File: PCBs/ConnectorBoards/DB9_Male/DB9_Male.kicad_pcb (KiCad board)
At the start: 2 copper layers, 4 parts, among them J1 DB9_Male, J2 Conn_02x05_Odd_Even

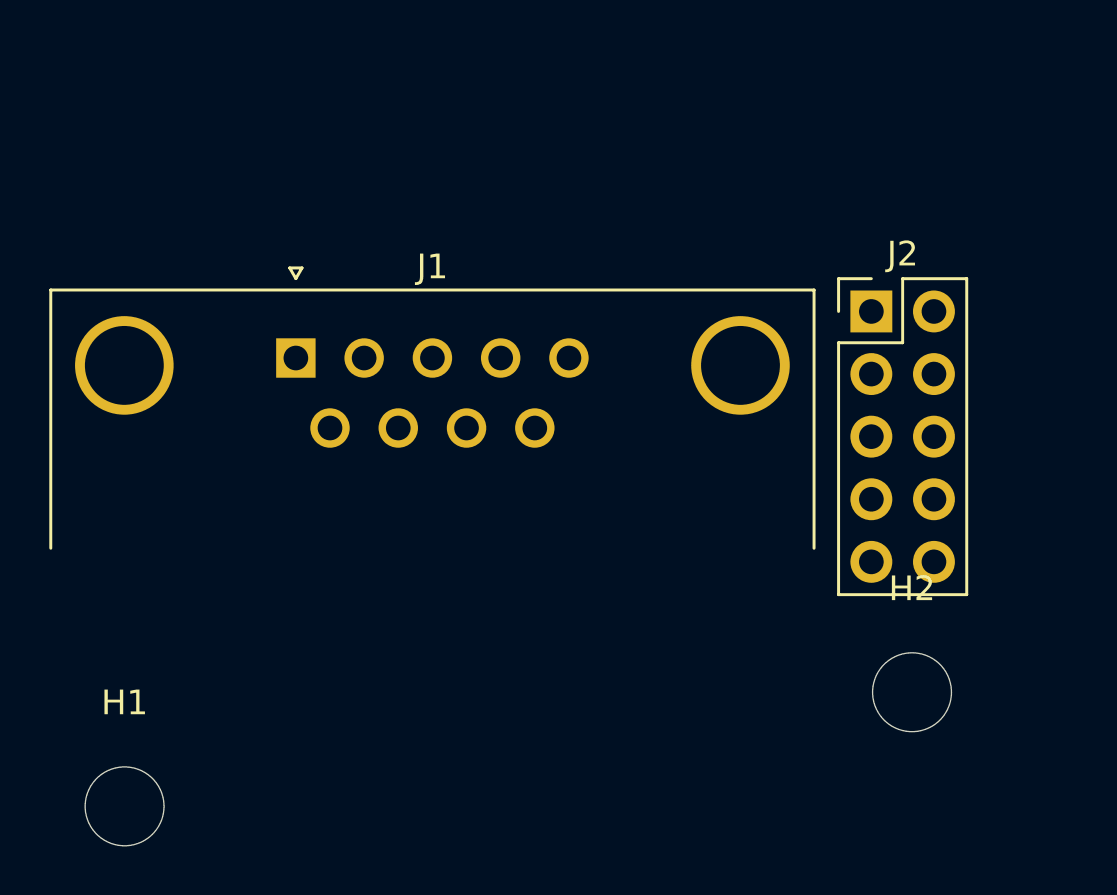
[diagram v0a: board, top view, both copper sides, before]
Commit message: generated the male pcbs
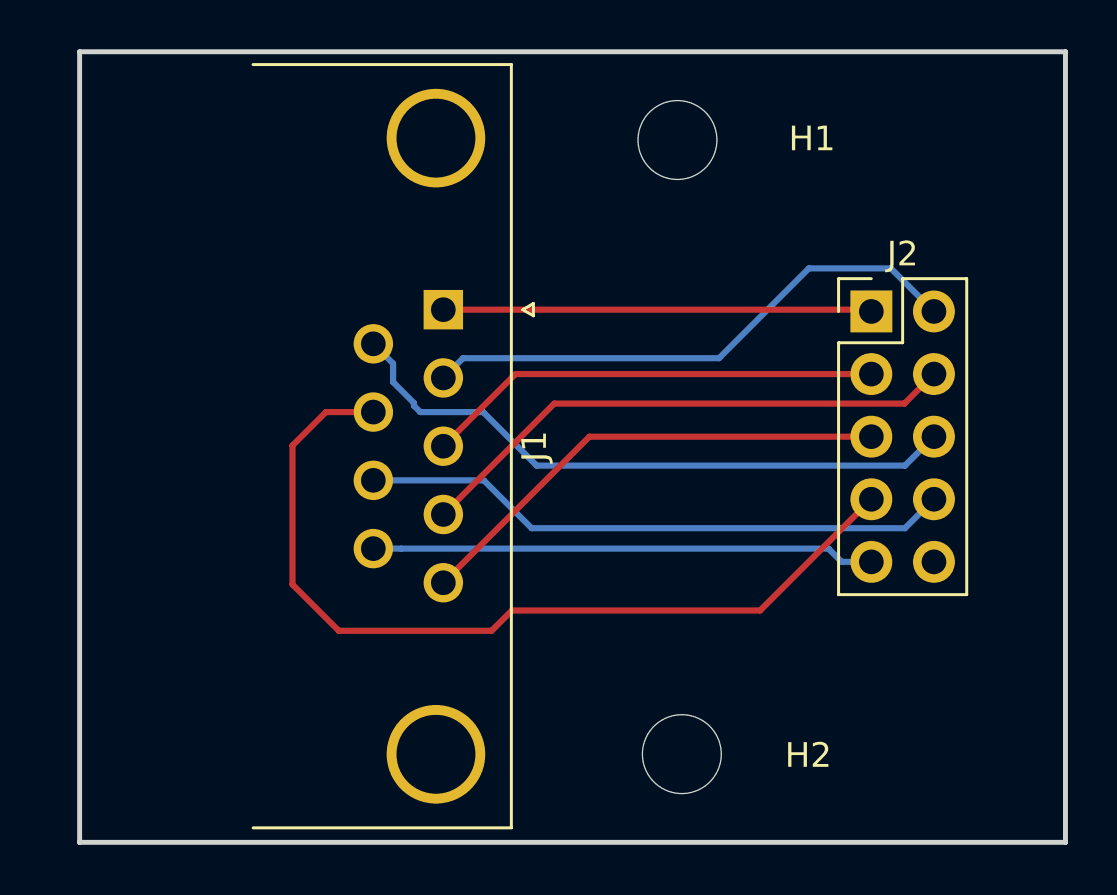
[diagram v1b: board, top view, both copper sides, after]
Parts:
- moved H1 35.1 mm to (167.1, 41.5)
- moved H2 9.67 mm to (167.3, 66.4)
- moved J1 6.30 mm to (157.6, 48.4), turned to 270 degrees
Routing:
- net 7: track 0.00 -> 36.0 mm
- net 6: track 0.00 -> 25.8 mm
- net 8: track 0.00 -> 24.0 mm
- net 2: track 0.00 -> 22.5 mm
- net 4: track 0.00 -> 22.3 mm
- net 9: track 0.00 -> 20.4 mm
- net 5: track 0.00 -> 19.8 mm
- net 3: track 0.00 -> 18.6 mm
- net 1: track 0.00 -> 17.4 mm
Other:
- board outline added: 40 x 32.1 mm
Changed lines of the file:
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@@
   (general
     (thickness 1.6)
-    (drawings 0)
-    (tracks 0)
+    (drawings 4)
+    (tracks 39)
     (zones 0)
     (modules 4)
@@
       (outputformat 1)
       (mirror false)
-      (drillshape 1)
+      (drillshape 0)
       (scaleselection 1)
-      (outputdirectory ""))
+      (outputdirectory "gerbers/"))
   )
   (net 0 "")
@@
   )
   (module MountingHole:MountingHole_3.2mm_M3 (layer F.Cu)
-    (at 144.673601 68.539401)
+    (at 167.1066 41.5036)
     (descr "Mounting Hole 3.2mm, no annular, M3")
     (tags "mounting hole 3.2mm no annular m3")
     (attr virtual)
-    (fp_text reference H1 (at 0 -4.2) (layer F.SilkS)
+    (fp_text reference H1 (at 5.461 -0.0508) (layer F.SilkS)
       (effects (font (size 1 1) (thickness 0.15)))
     )
@@
   )
   (module MountingHole:MountingHole_3.2mm_M3 (layer F.Cu)
-    (at 176.623601 63.909401)
+    (at 167.2844 66.421)
     (descr "Mounting Hole 3.2mm, no annular, M3")
     (tags "mounting hole 3.2mm no annular m3")
     (attr virtual)
-    (fp_text reference H2 (at 0 -4.2) (layer F.SilkS)
+    (fp_text reference H2 (at 5.1308 0.0508) (layer F.SilkS)
       (effects (font (size 1 1) (thickness 0.15)))
     )
@@
   )
   (module Connector_Dsub:DSUB-9_Male_Horizontal_P2.77x2.84mm_EdgePinOffset4.94mm_Housed_MountingHolesOffset7.48mm (layer F.Cu)
-    (at 151.623601 50.348739)
+    (at 157.607 48.387 270)
     (descr "9-pin D-Sub connector, horizontal/angled (90 deg), THT-mount, male, pitch 2.77x2.84mm, pin-PCB-offset 4.9399999999999995mm, distance of mounting holes 25mm, distance of mounting holes to PCB edge 7.4799999999999995mm, see https://disti-assets.s3.amazonaws.com/tonar/files/datasheets/16730.pdf")
     (tags "9-pin D-Sub connector horizontal angled 90deg THT male pitch 2.77x2.84mm pin-PCB-offset 4.9399999999999995mm mounting-holes-distance 25mm mounting-hole-offset 25mm")
-    (fp_text reference J1 (at 5.54 -3.7) (layer F.SilkS)
-      (effects (font (size 1 1) (thickness 0.15)))
-    )
-    (fp_text value DB9_Male (at 5.54 15.68) (layer F.Fab)
+    (fp_text reference J1 (at 5.54 -3.7 270) (layer F.SilkS)
+      (effects (font (size 1 1) (thickness 0.15)))
+    )
+    (fp_text value DB9_Male (at 5.54 15.68 270) (layer F.Fab)
       (effects (font (size 1 1) (thickness 0.15)))
     )
@@
     (fp_line (start 21.5 14.7) (end 21.5 -3.25) (layer F.CrtYd) (width 0.05))
     (fp_line (start 21.5 -3.25) (end -10.4 -3.25) (layer F.CrtYd) (width 0.05))
-    (fp_text user %R (at 5.54 11.18) (layer F.Fab)
-      (effects (font (size 1 1) (thickness 0.15)))
-    )
-    (pad 1 thru_hole rect (at 0 0) (size 1.6 1.6) (drill 1) (layers *.Cu *.Mask)
+    (fp_text user %R (at 5.54 11.18 270) (layer F.Fab)
+      (effects (font (size 1 1) (thickness 0.15)))
+    )
+    (pad 1 thru_hole rect (at 0 0 270) (size 1.6 1.6) (drill 1) (layers *.Cu *.Mask)
       (net 1 1))
-    (pad 2 thru_hole circle (at 2.77 0) (size 1.6 1.6) (drill 1) (layers *.Cu *.Mask)
+    (pad 2 thru_hole circle (at 2.77 0 270) (size 1.6 1.6) (drill 1) (layers *.Cu *.Mask)
       (net 2 2))
-    (pad 3 thru_hole circle (at 5.54 0) (size 1.6 1.6) (drill 1) (layers *.Cu *.Mask)
+    (pad 3 thru_hole circle (at 5.54 0 270) (size 1.6 1.6) (drill 1) (layers *.Cu *.Mask)
       (net 3 3))
-    (pad 4 thru_hole circle (at 8.31 0) (size 1.6 1.6) (drill 1) (layers *.Cu *.Mask)
+    (pad 4 thru_hole circle (at 8.31 0 270) (size 1.6 1.6) (drill 1) (layers *.Cu *.Mask)
       (net 4 4))
-    (pad 5 thru_hole circle (at 11.08 0) (size 1.6 1.6) (drill 1) (layers *.Cu *.Mask)
+    (pad 5 thru_hole circle (at 11.08 0 270) (size 1.6 1.6) (drill 1) (layers *.Cu *.Mask)
       (net 5 5))
-    (pad 6 thru_hole circle (at 1.385 2.84) (size 1.6 1.6) (drill 1) (layers *.Cu *.Mask)
+    (pad 6 thru_hole circle (at 1.385 2.84 270) (size 1.6 1.6) (drill 1) (layers *.Cu *.Mask)
       (net 6 6))
-    (pad 7 thru_hole circle (at 4.155 2.84) (size 1.6 1.6) (drill 1) (layers *.Cu *.Mask)
+    (pad 7 thru_hole circle (at 4.155 2.84 270) (size 1.6 1.6) (drill 1) (layers *.Cu *.Mask)
       (net 7 7))
-    (pad 8 thru_hole circle (at 6.925 2.84) (size 1.6 1.6) (drill 1) (layers *.Cu *.Mask)
+    (pad 8 thru_hole circle (at 6.925 2.84 270) (size 1.6 1.6) (drill 1) (layers *.Cu *.Mask)
       (net 8 8))
-    (pad 9 thru_hole circle (at 9.695 2.84) (size 1.6 1.6) (drill 1) (layers *.Cu *.Mask)
+    (pad 9 thru_hole circle (at 9.695 2.84 270) (size 1.6 1.6) (drill 1) (layers *.Cu *.Mask)
       (net 9 9))
-    (pad 0 thru_hole circle (at -6.96 0.3) (size 4 4) (drill 3.2) (layers *.Cu *.Mask))
-    (pad 0 thru_hole circle (at 18.04 0.3) (size 4 4) (drill 3.2) (layers *.Cu *.Mask))
+    (pad 0 thru_hole circle (at -6.96 0.3 270) (size 4 4) (drill 3.2) (layers *.Cu *.Mask))
+    (pad 0 thru_hole circle (at 18.04 0.3 270) (size 4 4) (drill 3.2) (layers *.Cu *.Mask))
     (model ${KISYS3DMOD}/Connector_Dsub.3dshapes/DSUB-9_Male_Horizontal_P2.77x2.84mm_EdgePinOffset4.94mm_Housed_MountingHolesOffset7.48mm.wrl
       (at (xyz 0 0 0))
@@
     )
   )
+  (gr_line (start 142.8496 37.9222) (end 142.8496 70) (layer Edge.Cuts) (width 0.2))
+  (gr_line (start 182.8496 37.9222) (end 142.8496 37.9222) (layer Edge.Cuts) (width 0.2))
+  (gr_line (start 182.8496 70) (end 182.8496 37.9222) (layer Edge.Cuts) (width 0.2))
+  (gr_line (start 142.8496 70) (end 182.8496 70) (layer Edge.Cuts) (width 0.2))
+  (segment (start 174.9012 48.387) (end 174.973601 48.459401) (width 0.25) (layer F.Cu) (net 1))
+  (segment (start 157.607 48.387) (end 174.9012 48.387) (width 0.25) (layer F.Cu) (net 1))
+  (segment (start 158.406999 50.357001) (end 168.794199 50.357001) (width 0.25) (layer B.Cu) (net 2))
+  (segment (start 157.607 51.157) (end 158.406999 50.357001) (width 0.25) (layer B.Cu) (net 2))
+  (segment (start 168.794199 50.357001) (end 172.4406 46.7106) (width 0.25) (layer B.Cu) (net 2))
+  (segment (start 175.7648 46.7106) (end 177.513601 48.459401) (width 0.25) (layer B.Cu) (net 2))
+  (segment (start 172.4406 46.7106) (end 175.7648 46.7106) (width 0.25) (layer B.Cu) (net 2))
+  (segment (start 160.534599 50.999401) (end 157.607 53.927) (width 0.25) (layer F.Cu) (net 3))
+  (segment (start 174.973601 50.999401) (end 160.534599 50.999401) (width 0.25) (layer F.Cu) (net 3))
+  (segment (start 157.607 56.697) (end 162.107 52.197) (width 0.25) (layer F.Cu) (net 4))
+  (segment (start 176.316002 52.197) (end 177.513601 50.999401) (width 0.25) (layer F.Cu) (net 4))
+  (segment (start 162.107 52.197) (end 176.316002 52.197) (width 0.25) (layer F.Cu) (net 4))
+  (segment (start 163.534599 53.539401) (end 157.607 59.467) (width 0.25) (layer F.Cu) (net 5))
+  (segment (start 174.973601 53.539401) (end 163.534599 53.539401) (width 0.25) (layer F.Cu) (net 5))
+  (segment (start 159.221398 52.541398) (end 161.394402 54.714402) (width 0.25) (layer B.Cu) (net 6))
+  (segment (start 156.672597 52.541398) (end 159.221398 52.541398) (width 0.25) (layer B.Cu) (net 6))
+  (segment (start 176.3386 54.714402) (end 177.513601 53.539401) (width 0.25) (layer B.Cu) (net 6))
+  (segment (start 156.4132 52.282001) (end 156.672597 52.541398) (width 0.25) (layer B.Cu) (net 6))
+  (segment (start 161.394402 54.714402) (end 176.3386 54.714402) (width 0.25) (layer B.Cu) (net 6))
+  (segment (start 154.767 49.772) (end 155.566999 50.571999) (width 0.25) (layer B.Cu) (net 6))
+  (segment (start 155.566999 50.571999) (end 155.566999 51.325399) (width 0.25) (layer B.Cu) (net 6))
+  (segment (start 155.566999 51.325399) (end 156.4132 52.1716) (width 0.25) (layer B.Cu) (net 6))
+  (segment (start 156.4132 52.1716) (end 156.4132 52.282001) (width 0.25) (layer B.Cu) (net 6))
+  (segment (start 170.461001 60.592001) (end 160.387999 60.592001) (width 0.25) (layer F.Cu) (net 7))
+  (segment (start 174.973601 56.079401) (end 170.461001 60.592001) (width 0.25) (layer F.Cu) (net 7))
+  (segment (start 160.387999 60.592001) (end 159.5628 61.4172) (width 0.25) (layer F.Cu) (net 7))
+  (segment (start 159.5628 61.4172) (end 153.3652 61.4172) (width 0.25) (layer F.Cu) (net 7))
+  (segment (start 153.3652 61.4172) (end 151.4856 59.5376) (width 0.25) (layer F.Cu) (net 7))
+  (segment (start 151.4856 59.5376) (end 151.4856 53.8988) (width 0.25) (layer F.Cu) (net 7))
+  (segment (start 152.8424 52.542) (end 154.767 52.542) (width 0.25) (layer F.Cu) (net 7))
+  (segment (start 151.4856 53.8988) (end 152.8424 52.542) (width 0.25) (layer F.Cu) (net 7))
+  (segment (start 176.3386 57.254402) (end 161.191202 57.254402) (width 0.25) (layer B.Cu) (net 8))
+  (segment (start 177.513601 56.079401) (end 176.3386 57.254402) (width 0.25) (layer B.Cu) (net 8))
+  (segment (start 159.2488 55.312) (end 154.767 55.312) (width 0.25) (layer B.Cu) (net 8))
+  (segment (start 161.191202 57.254402) (end 159.2488 55.312) (width 0.25) (layer B.Cu) (net 8))
+  (segment (start 155.89837 58.082) (end 154.767 58.082) (width 0.25) (layer B.Cu) (net 9))
+  (segment (start 173.77152 58.619401) (end 173.234119 58.082) (width 0.25) (layer B.Cu) (net 9))
+  (segment (start 173.234119 58.082) (end 155.89837 58.082) (width 0.25) (layer B.Cu) (net 9))
+  (segment (start 174.973601 58.619401) (end 173.77152 58.619401) (width 0.25) (layer B.Cu) (net 9))
 )
